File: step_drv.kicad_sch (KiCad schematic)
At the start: 64 parts, among them J17 X-STEPPER, J18 Y-STEPPER, J19 ZA-STEPPER, J20 E0-STEPPER, J21 ZB-STEPPER, U6 TMC2226-SA-T, U7 TMC2226-SA-T, U8 TMC2226-SA-T, U9 TMC2226-SA-T

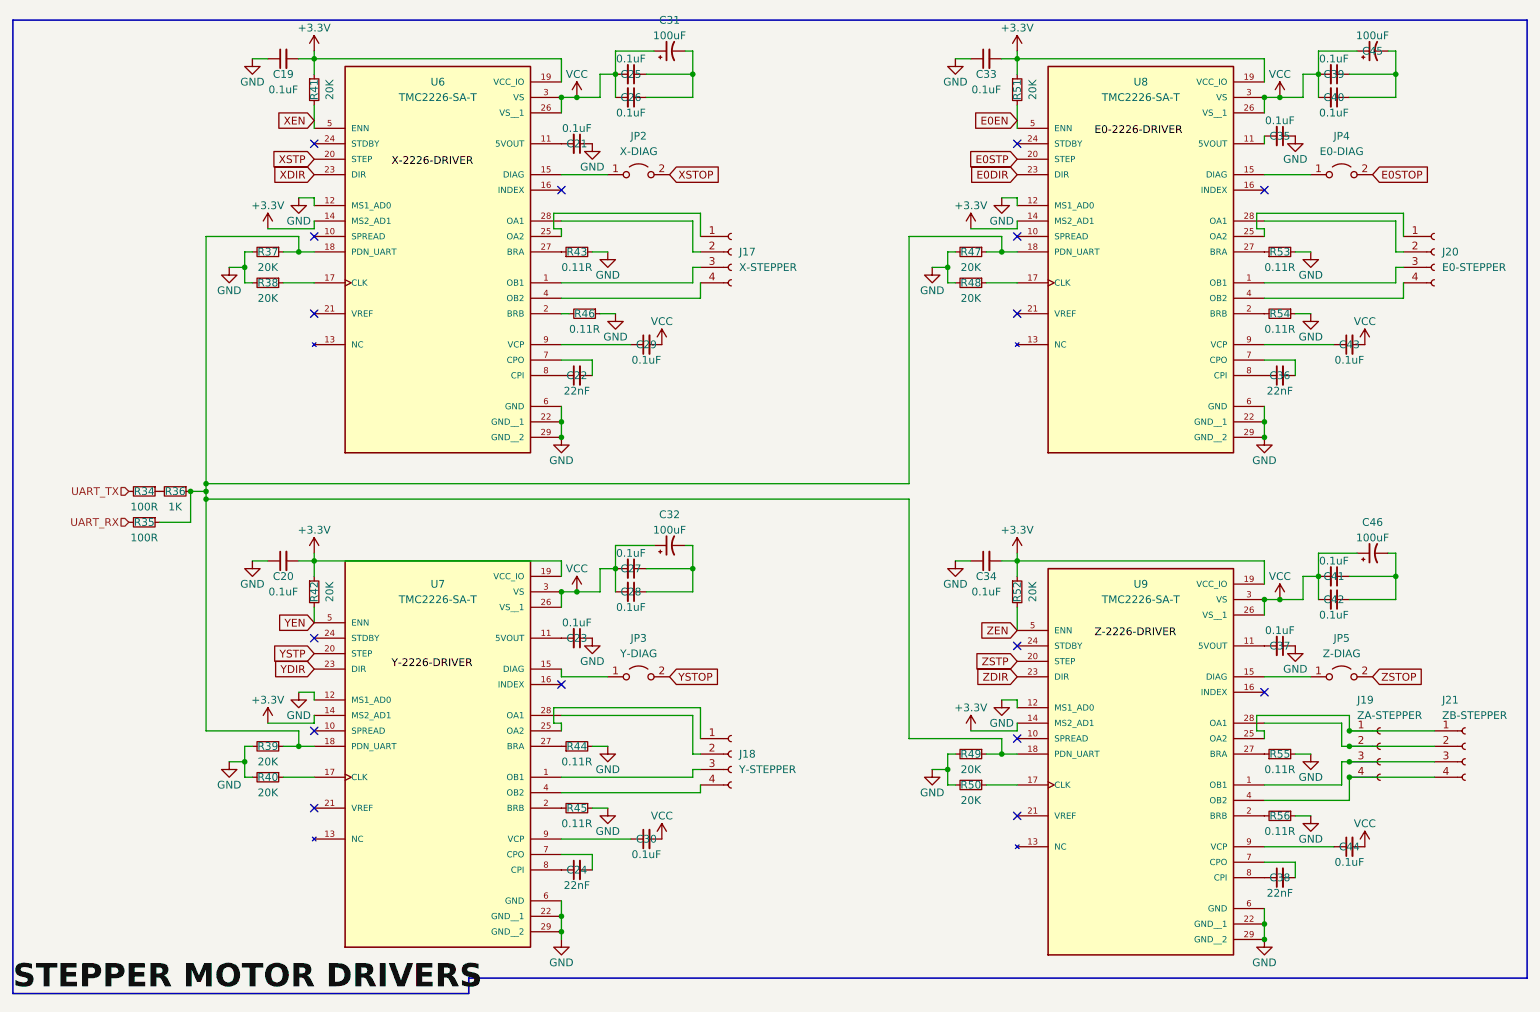
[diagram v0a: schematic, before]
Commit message: finished, for now, finally
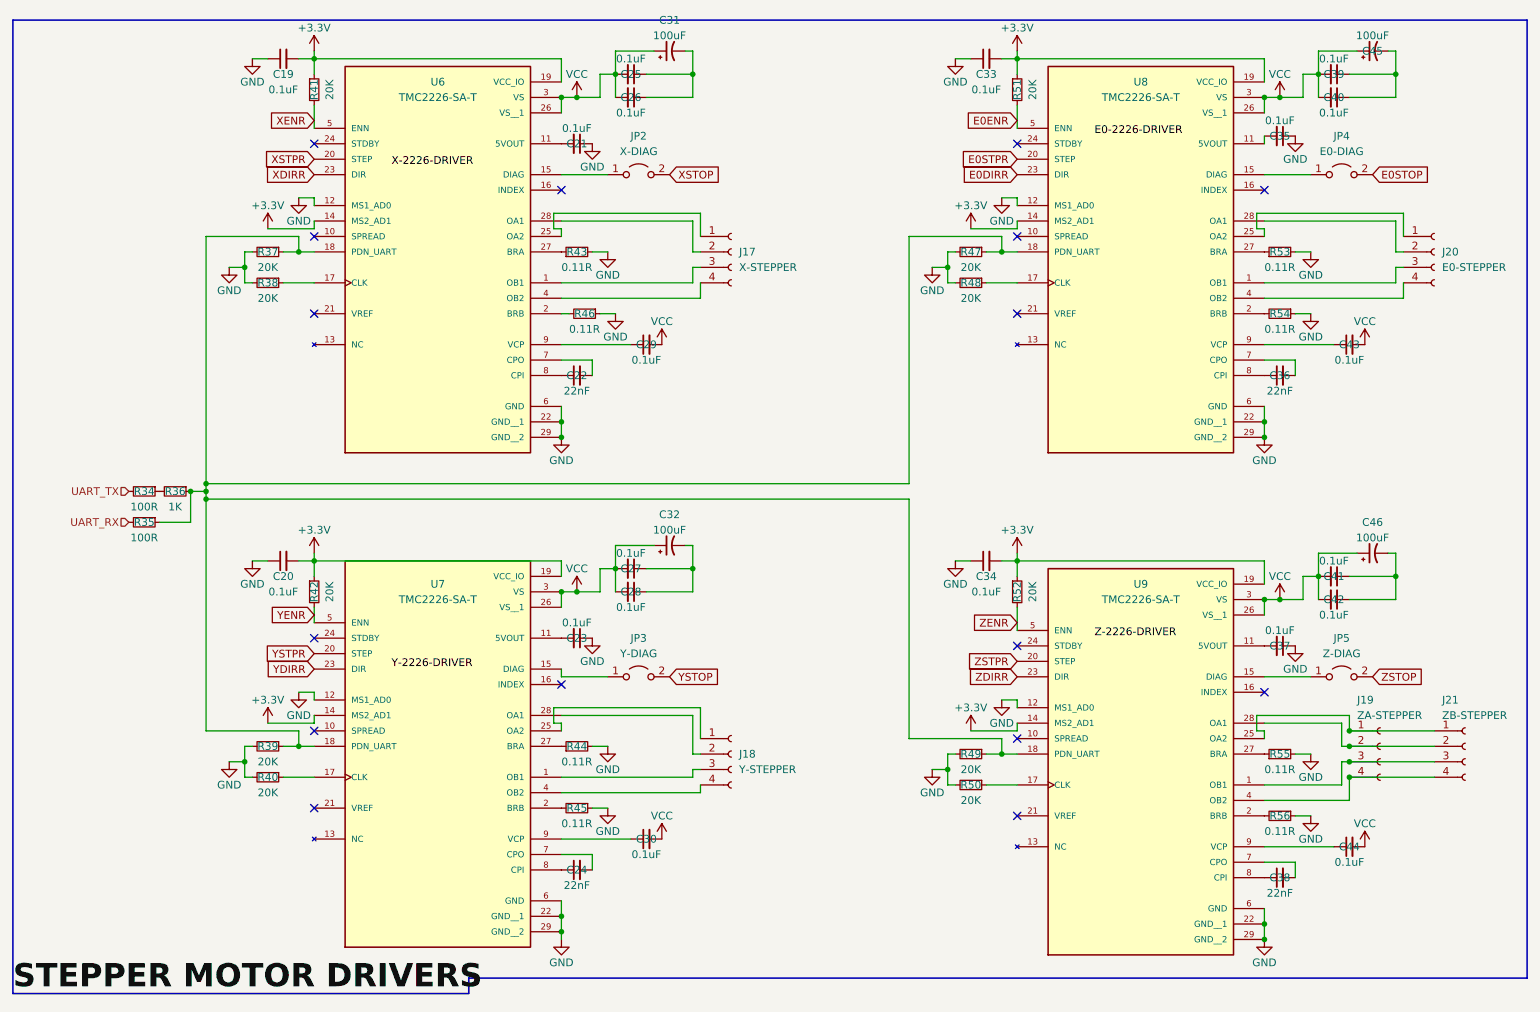
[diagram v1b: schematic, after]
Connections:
- net E0DIR renamed E0DIRR
- net E0EN renamed E0ENR
- net E0STP renamed E0STPR
- net XDIR renamed XDIRR
- net XEN renamed XENR
- net XSTP renamed XSTPR
- net YDIR renamed YDIRR
- net YEN renamed YENR
- net YSTP renamed YSTPR
- net ZDIR renamed ZDIRR
- net ZEN renamed ZENR
- net ZSTP renamed ZSTPR
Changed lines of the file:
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@@
     (effects (font (size 1.27 1.27)) (justify left bottom))
-  )
-  (global_label "XEN" (shape input) (at 64.77 30.48 180) (fields_autoplaced)
-    (effects (font (size 1.27 1.27)) (justify right))
-    (property "Intersheet References" "${INTERSHEET_REFS}" (id 0) (at 58.6679 30.4006 0)
-      (effects (font (size 1.27 1.27)) (justify right) hide)
-    )
-  )
-  (global_label "E0STP" (shape input) (at 180.34 36.83 180) (fields_autoplaced)
-    (effects (font (size 1.27 1.27)) (justify right))
-    (property "Intersheet References" "${INTERSHEET_REFS}" (id 0) (at 172.1212 36.7506 0)
-      (effects (font (size 1.27 1.27)) (justify right) hide)
-    )
   )
   (global_label "XSTOP" (shape input) (at 123.19 39.37 0) (fields_autoplaced)
@@
     )
   )
-  (global_label "ZSTP" (shape input) (at 180.34 119.38 180) (fields_autoplaced)
+  (global_label "YSTPR" (shape input) (at 64.77 118.11 180) (fields_autoplaced)
     (effects (font (size 1.27 1.27)) (justify right))
-    (property "Intersheet References" "${INTERSHEET_REFS}" (id 0) (at 173.2702 119.3006 0)
-      (effects (font (size 1.27 1.27)) (justify right) hide)
-    )
-  )
-  (global_label "YEN" (shape input) (at 64.77 113.03 180) (fields_autoplaced)
-    (effects (font (size 1.27 1.27)) (justify right))
-    (property "Intersheet References" "${INTERSHEET_REFS}" (id 0) (at 58.7888 112.9506 0)
+    (property "Intersheet References" "${INTERSHEET_REFS}" (id 0) (at 56.5512 118.1894 0)
       (effects (font (size 1.27 1.27)) (justify right) hide)
     )
@@
     )
   )
-  (global_label "ZDIR" (shape input) (at 180.34 121.92 180) (fields_autoplaced)
+  (global_label "ZENR" (shape input) (at 180.34 113.03 180) (fields_autoplaced)
     (effects (font (size 1.27 1.27)) (justify right))
-    (property "Intersheet References" "${INTERSHEET_REFS}" (id 0) (at 173.5726 121.8406 0)
+    (property "Intersheet References" "${INTERSHEET_REFS}" (id 0) (at 172.9679 113.1094 0)
+      (effects (font (size 1.27 1.27)) (justify right) hide)
+    )
+  )
+  (global_label "XENR" (shape input) (at 64.77 30.48 180) (fields_autoplaced)
+    (effects (font (size 1.27 1.27)) (justify right))
+    (property "Intersheet References" "${INTERSHEET_REFS}" (id 0) (at 57.3979 30.5594 0)
+      (effects (font (size 1.27 1.27)) (justify right) hide)
+    )
+  )
+  (global_label "XDIRR" (shape input) (at 64.77 39.37 180) (fields_autoplaced)
+    (effects (font (size 1.27 1.27)) (justify right))
+    (property "Intersheet References" "${INTERSHEET_REFS}" (id 0) (at 56.7326 39.4494 0)
+      (effects (font (size 1.27 1.27)) (justify right) hide)
+    )
+  )
+  (global_label "ZSTPR" (shape input) (at 180.34 119.38 180) (fields_autoplaced)
+    (effects (font (size 1.27 1.27)) (justify right))
+    (property "Intersheet References" "${INTERSHEET_REFS}" (id 0) (at 172.0002 119.4594 0)
+      (effects (font (size 1.27 1.27)) (justify right) hide)
+    )
+  )
+  (global_label "E0ENR" (shape input) (at 180.34 30.48 180) (fields_autoplaced)
+    (effects (font (size 1.27 1.27)) (justify right))
+    (property "Intersheet References" "${INTERSHEET_REFS}" (id 0) (at 171.8188 30.5594 0)
       (effects (font (size 1.27 1.27)) (justify right) hide)
     )
@@
     )
   )
-  (global_label "ZEN" (shape input) (at 180.34 114.3 180) (fields_autoplaced)
+  (global_label "ZDIRR" (shape input) (at 180.34 121.92 180) (fields_autoplaced)
     (effects (font (size 1.27 1.27)) (justify right))
-    (property "Intersheet References" "${INTERSHEET_REFS}" (id 0) (at 174.2379 114.2206 0)
+    (property "Intersheet References" "${INTERSHEET_REFS}" (id 0) (at 172.3026 121.9994 0)
       (effects (font (size 1.27 1.27)) (justify right) hide)
     )
   )
-  (global_label "YSTP" (shape input) (at 64.77 118.11 180) (fields_autoplaced)
+  (global_label "E0DIRR" (shape input) (at 180.34 39.37 180) (fields_autoplaced)
     (effects (font (size 1.27 1.27)) (justify right))
-    (property "Intersheet References" "${INTERSHEET_REFS}" (id 0) (at 57.8212 118.0306 0)
+    (property "Intersheet References" "${INTERSHEET_REFS}" (id 0) (at 171.1536 39.4494 0)
       (effects (font (size 1.27 1.27)) (justify right) hide)
     )
   )
-  (global_label "YDIR" (shape input) (at 64.77 120.65 180) (fields_autoplaced)
+  (global_label "XSTPR" (shape input) (at 64.77 36.83 180) (fields_autoplaced)
     (effects (font (size 1.27 1.27)) (justify right))
-    (property "Intersheet References" "${INTERSHEET_REFS}" (id 0) (at 58.1236 120.5706 0)
+    (property "Intersheet References" "${INTERSHEET_REFS}" (id 0) (at 56.4302 36.9094 0)
       (effects (font (size 1.27 1.27)) (justify right) hide)
     )
   )
-  (global_label "E0DIR" (shape input) (at 180.34 39.37 180) (fields_autoplaced)
+  (global_label "E0STPR" (shape input) (at 180.34 36.83 180) (fields_autoplaced)
     (effects (font (size 1.27 1.27)) (justify right))
-    (property "Intersheet References" "${INTERSHEET_REFS}" (id 0) (at 172.4236 39.2906 0)
+    (property "Intersheet References" "${INTERSHEET_REFS}" (id 0) (at 170.8512 36.9094 0)
       (effects (font (size 1.27 1.27)) (justify right) hide)
     )
   )
-  (global_label "E0EN" (shape input) (at 180.34 30.48 180) (fields_autoplaced)
+  (global_label "YENR" (shape input) (at 64.77 111.76 180) (fields_autoplaced)
     (effects (font (size 1.27 1.27)) (justify right))
-    (property "Intersheet References" "${INTERSHEET_REFS}" (id 0) (at 173.0888 30.4006 0)
+    (property "Intersheet References" "${INTERSHEET_REFS}" (id 0) (at 57.5188 111.8394 0)
       (effects (font (size 1.27 1.27)) (justify right) hide)
     )
   )
-  (global_label "XSTP" (shape input) (at 64.77 36.83 180) (fields_autoplaced)
+  (global_label "YDIRR" (shape input) (at 64.77 120.65 180) (fields_autoplaced)
     (effects (font (size 1.27 1.27)) (justify right))
-    (property "Intersheet References" "${INTERSHEET_REFS}" (id 0) (at 57.7002 36.7506 0)
+    (property "Intersheet References" "${INTERSHEET_REFS}" (id 0) (at 56.8536 120.7294 0)
       (effects (font (size 1.27 1.27)) (justify right) hide)
     )
@@
     )
   )
-  (global_label "XDIR" (shape input) (at 64.77 39.37 180) (fields_autoplaced)
-    (effects (font (size 1.27 1.27)) (justify right))
-    (property "Intersheet References" "${INTERSHEET_REFS}" (id 0) (at 58.0026 39.2906 0)
-      (effects (font (size 1.27 1.27)) (justify right) hide)
-    )
-  )
